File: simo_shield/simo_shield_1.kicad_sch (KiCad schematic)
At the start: 6 parts, among them J1 CONECTOR DEBUG_UART, J2 VBAT, U1 YAAJ_BluePill_Part_Like_SWD_B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, U2 elemon_board, U3 flash_externa, U4 mpu6050

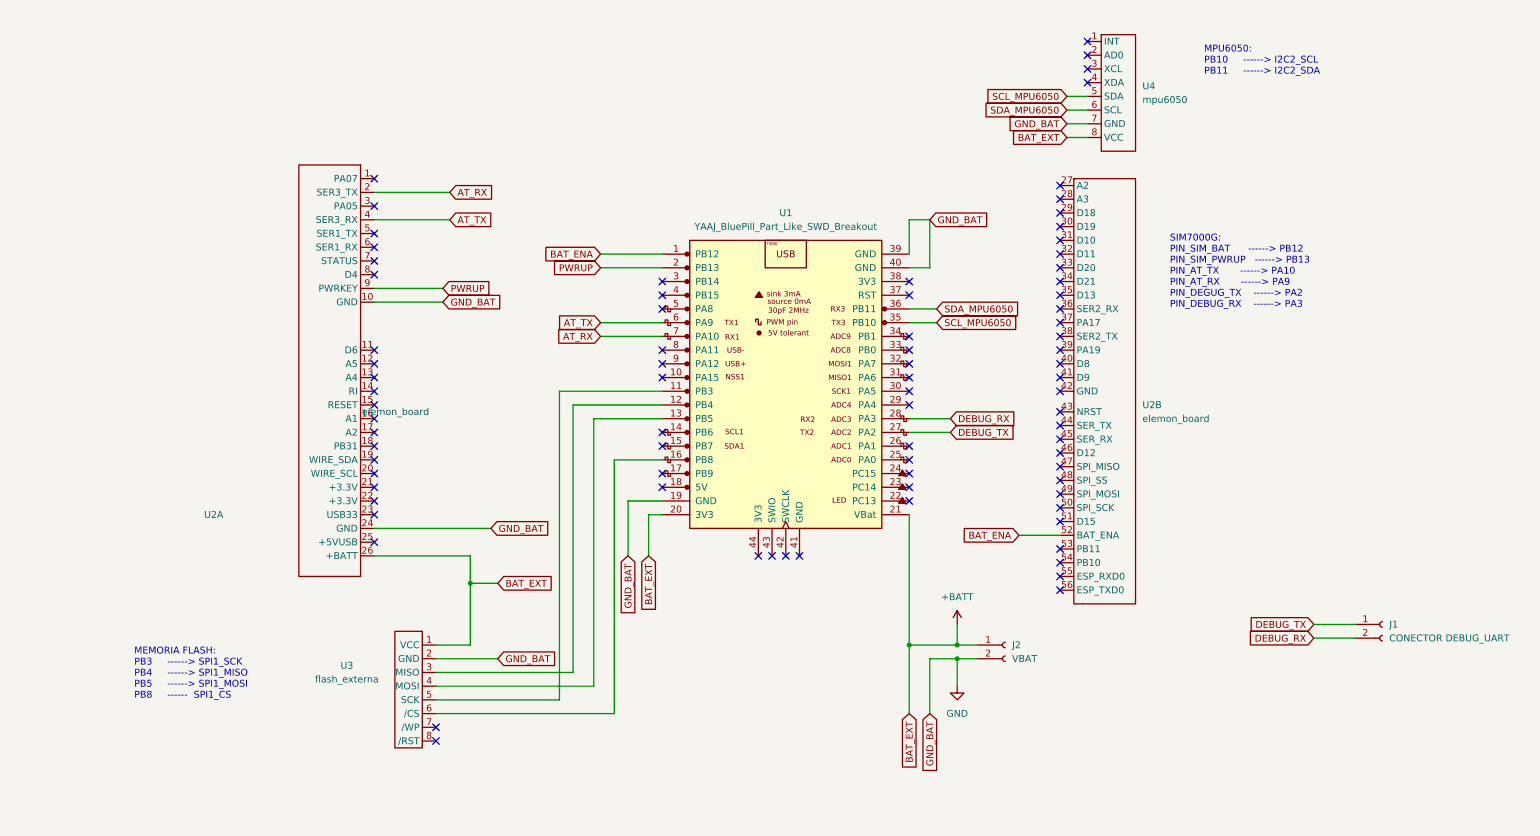
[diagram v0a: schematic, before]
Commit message: casi terminado, revisar PCB, error de conexion pero no entiendo por que.
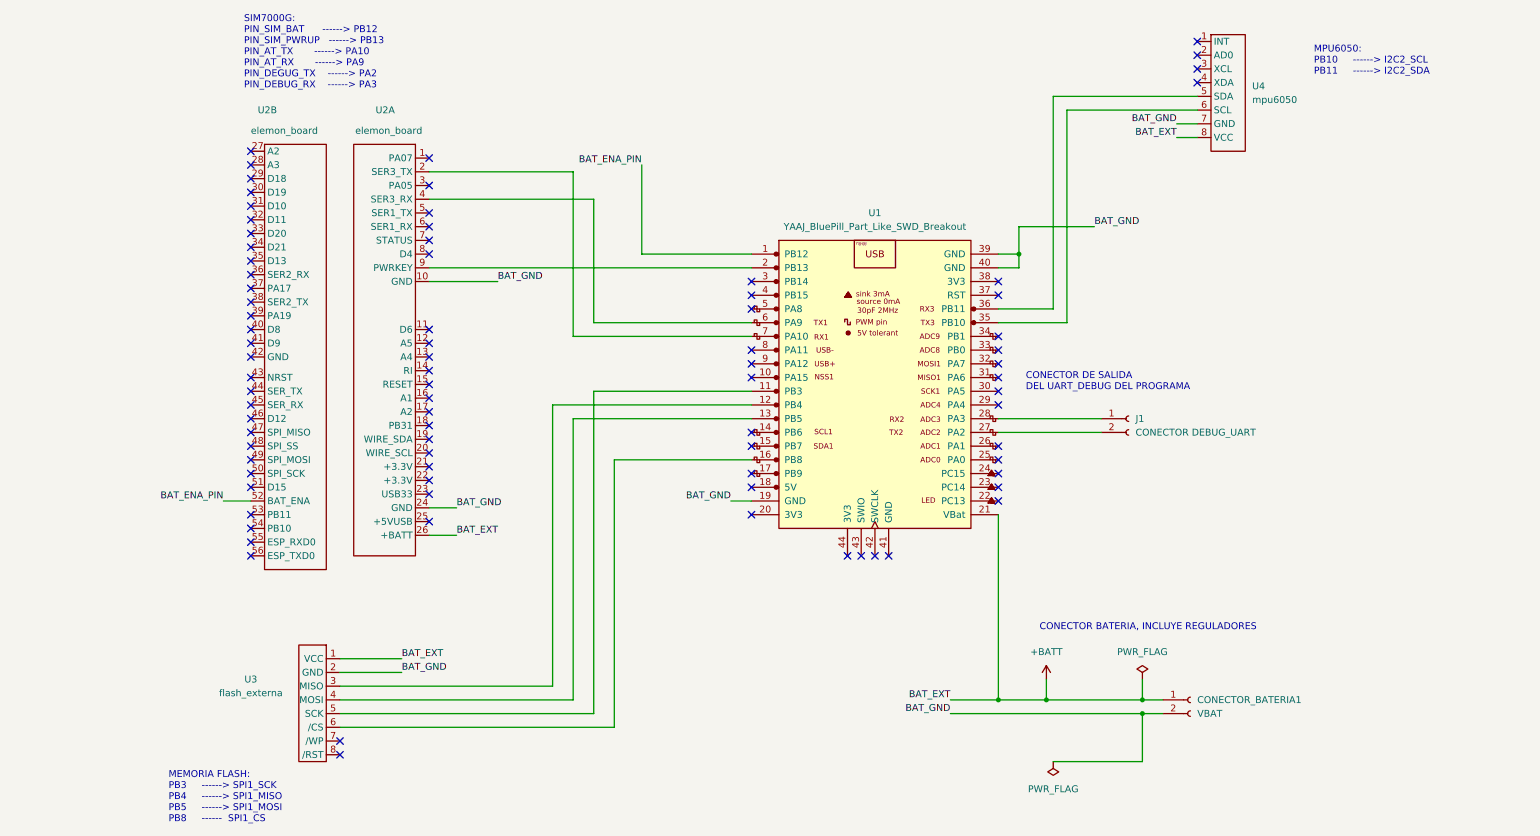
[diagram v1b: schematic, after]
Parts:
- U1: footprint simo:YAAJ_BluePill_SWD_1 -> bluepill:YAAJ_BluePill_SWD_1
- renumbered J2 to CONECTOR_BATERIA1
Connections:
- net +BATT: no longer U1.20 (3V3)
- net AT_RX: no longer names the net of U1.7 (PA10), U2.2 (SER3_TX)
- net AT_TX: no longer names the net of U1.6 (PA9), U2.4 (SER3_RX)
- net BAT_ENA renamed BAT_ENA_PIN
- net DEBUG_RX: no longer names the net of J1.2 (Pin_2)
- net DEBUG_RX: now also U1.27 (PA2); no longer U1.28 (PA3)
- net DEBUG_TX: no longer names the net of J1.1 (Pin_1)
- net DEBUG_TX: now also U1.28 (PA3); no longer U1.27 (PA2)
- net GND renamed BAT_GND
- net PWRUP: no longer names the net of U1.2 (PB13), U2.9 (PWRKEY)
- net SCL_MPU6050: no longer names the net of U1.35 (PB10)
- net SCL_MPU6050: now also U4.6 (SCL); no longer U4.5 (SDA)
- net SDA_MPU6050: no longer names the net of U1.36 (PB11)
- net SDA_MPU6050: now also U4.5 (SDA); no longer U4.6 (SCL)
- no-connect marks 82 -> 83
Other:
- note added: "CONECTOR BATERIA, INCLUYE REGULADORES"
- note added: "CONECTOR DE SALIDA DEL UART_DEBUG DEL PROGRAMA"
- moved on the sheet: CONECTOR_BATERIA1, J1, U1, U2A, U2B, U3, U4
